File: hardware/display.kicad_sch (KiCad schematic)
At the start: 6 parts, among them J1 Conn_02x10_Odd_Even_Shielded, J2 Conn_02x10_Odd_Even_Shielded

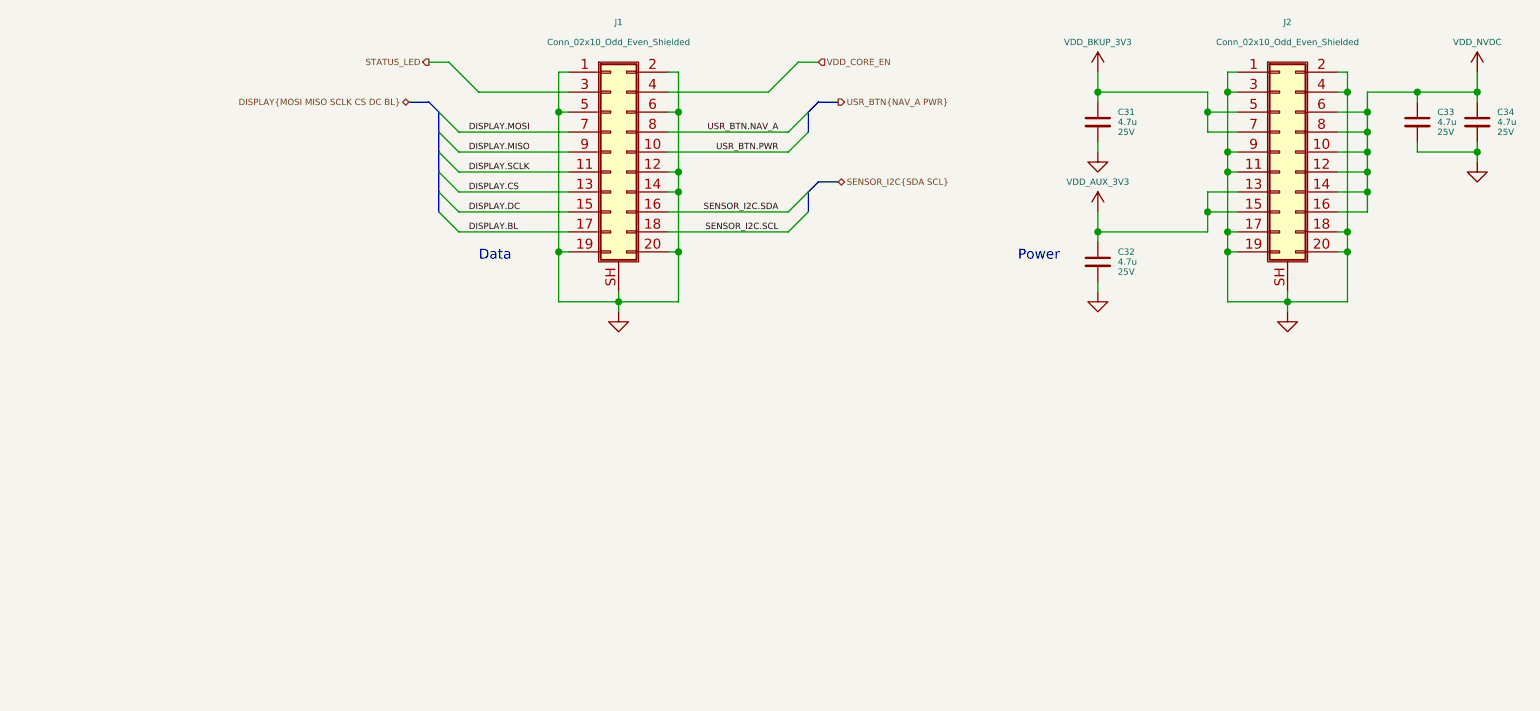
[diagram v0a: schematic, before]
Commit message: fixing submodule
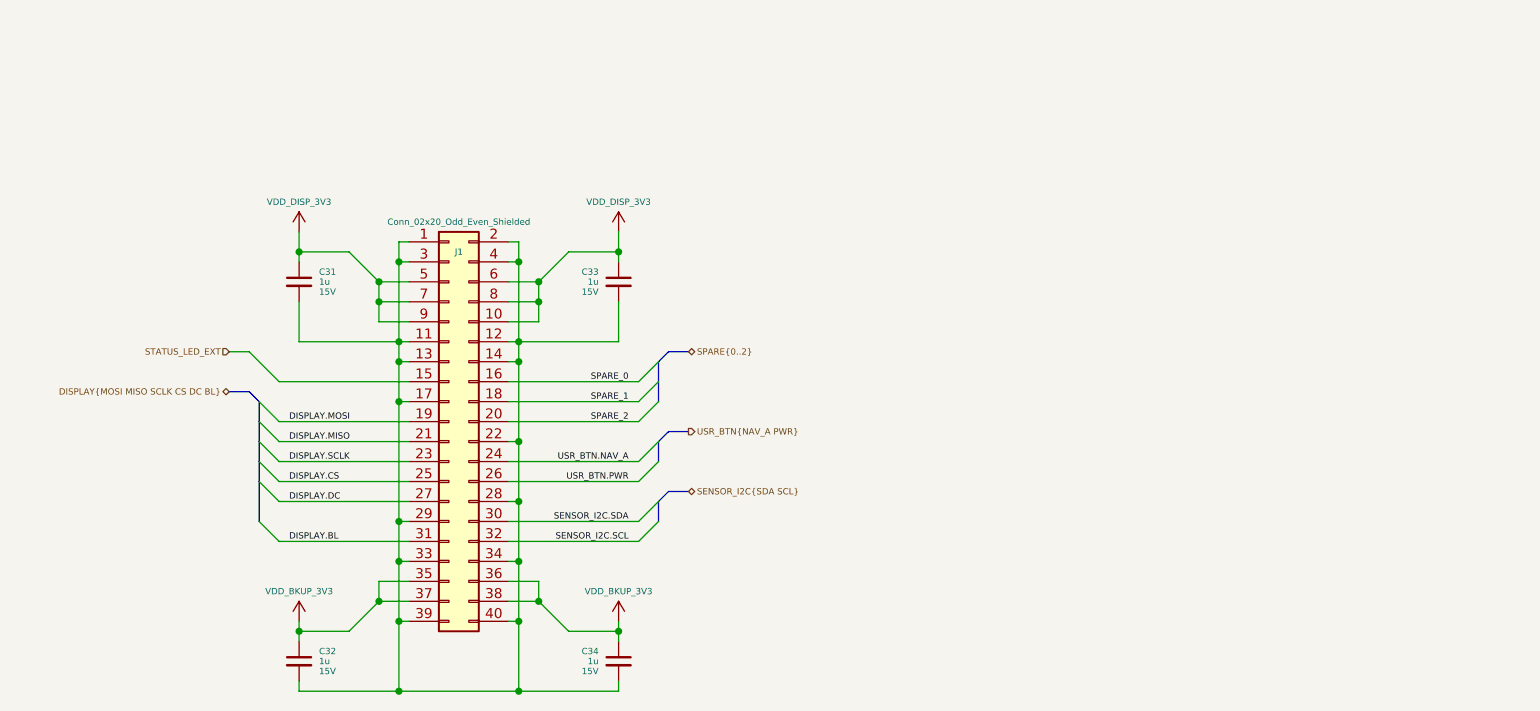
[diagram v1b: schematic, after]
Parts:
- removed J1, J2: Conn_02x10_Odd_Even_Shielded, Connector_Molex:Molex_SlimStack_55560-0201_2x10_P0.50mm_Vertical, symbol Connector_Generic_Shielded:Conn_02x10_Odd_Even_Shielded
- added J1: Conn_02x20_Odd_Even_Shielded, Connector_Molex:Molex_SlimStack_502426-4010_2x20_P0.40mm_Vertical, symbol Connector_Generic:Conn_02x20_Odd_Even
- C31, C32, C33, C34: value 4.7u -> 1u; Voltage 25V -> 15V
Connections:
- net VDD_AUX_3V3 is gone; now on net VCC_BKUP_3V3: C32.1
- net DISPLAY.BL: now also J1.31 (Pin_31)
- net DISPLAY.CS: now also J1.25 (Pin_25)
- net DISPLAY.DC: now also J1.27 (Pin_27)
- net DISPLAY.MISO: now also J1.21 (Pin_21)
- net DISPLAY.MOSI: now also J1.19 (Pin_19)
- net DISPLAY.SCLK: now also J1.23 (Pin_23)
- net SENSOR_I2C.SCL: now also J1.32 (Pin_32)
- net SENSOR_I2C.SDA: now also J1.30 (Pin_30)
- net USR_BTN.NAV_A: now also J1.24 (Pin_24)
- net USR_BTN.PWR: now also J1.26 (Pin_26)
- net VCC_BKUP_3V3: now also C34.1, J1.35 (Pin_35), J1.36 (Pin_36), J1.37 (Pin_37), J1.38 (Pin_38); no longer C31.1
- net GND: no longer names the net of C31.2, C32.2, C33.2, C34.2
- net GND: now also J1.1 (Pin_1), J1.11 (Pin_11), J1.12 (Pin_12), J1.13 (Pin_13), J1.14 (Pin_14), J1.17 (Pin_17), J1.2 (Pin_2), J1.22 (Pin_22), J1.28 (Pin_28), J1.29 (Pin_29), J1.3 (Pin_3), J1.33 (Pin_33), J1.34 (Pin_34), J1.39 (Pin_39), J1.4 (Pin_4), J1.40 (Pin_40)
- net VDD_NVDC renamed VDD_DISP_3V3
- net VDD_DISP_3V3: now also C31.1, J1.10 (Pin_10), J1.5 (Pin_5), J1.6 (Pin_6), J1.7 (Pin_7), J1.8 (Pin_8), J1.9 (Pin_9); no longer C34.1
- new net SPARE_0: J1.16 (Pin_16)
- new net SPARE_1: J1.18 (Pin_18)
- new net SPARE_2: J1.20 (Pin_20)
- new net STATUS_LED_EXT: J1.15 (Pin_15)
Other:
- note removed: "Data"
- note removed: "Power"
